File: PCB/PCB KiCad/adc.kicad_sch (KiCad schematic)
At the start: 10 parts, among them U2 NAU7802SGI, U4 LP5951MFX-1.8_NOPB

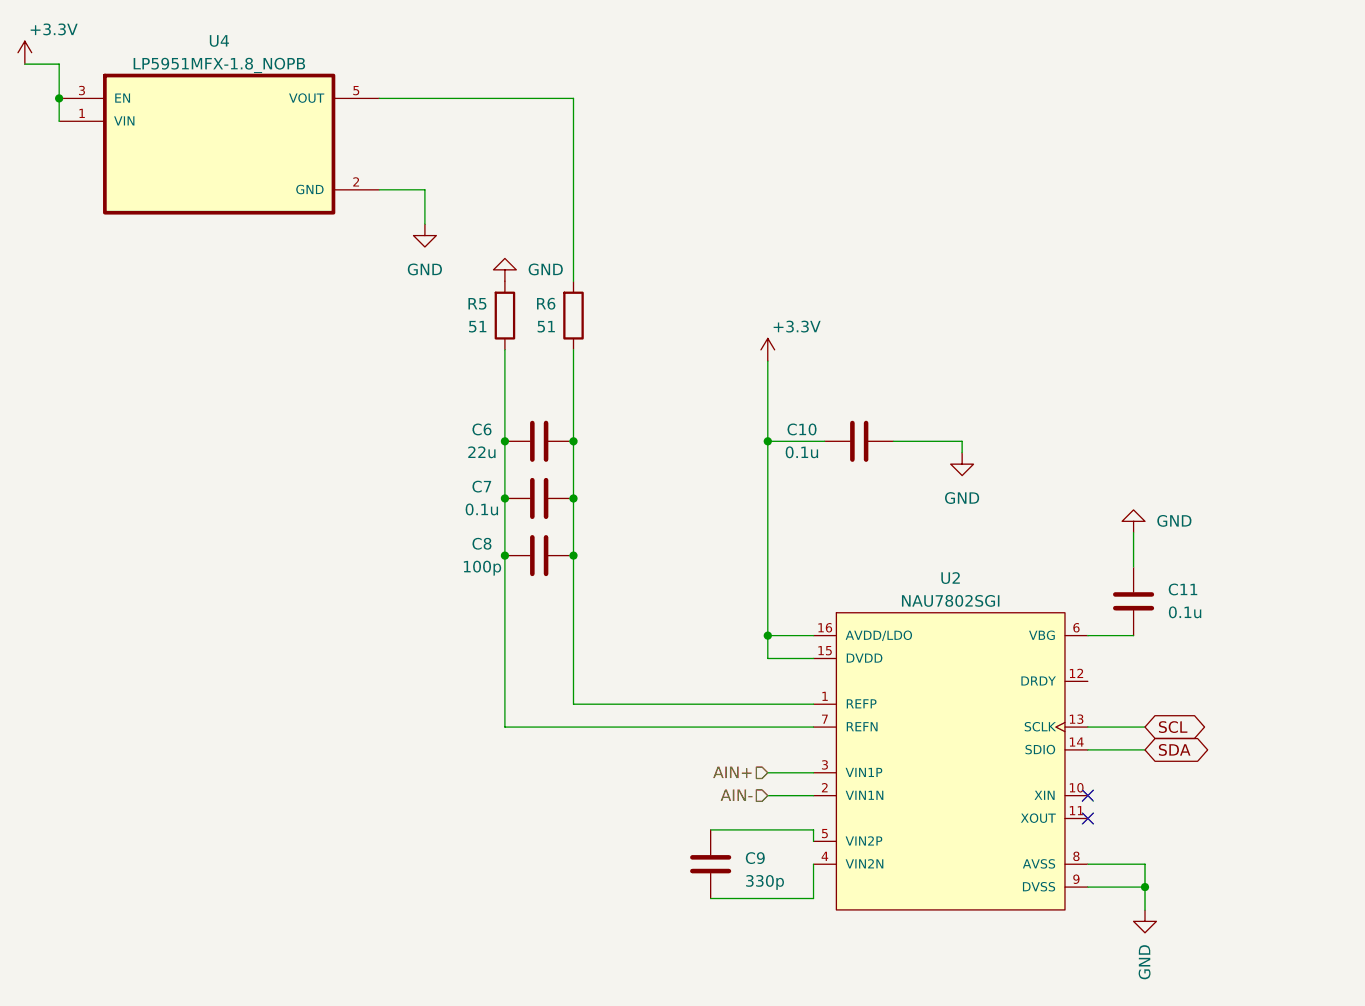
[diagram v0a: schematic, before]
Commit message: Minor schematic cleanup!
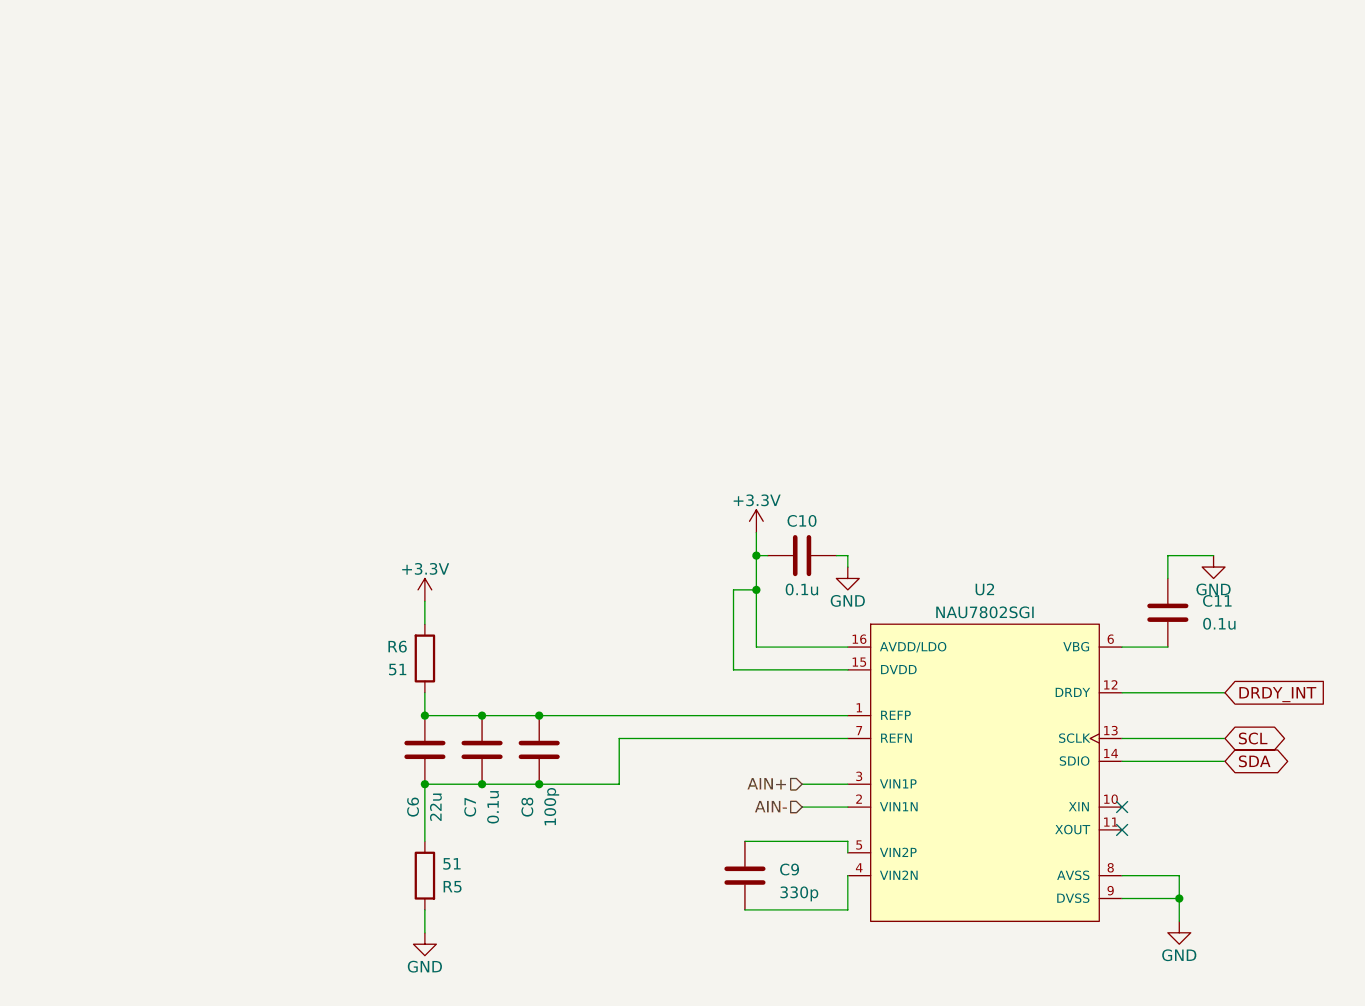
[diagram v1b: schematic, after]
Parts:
- removed U4: LP5951MFX-1.8_NOPB, LP5951MFX-1.8_NOPB:SOT95P280X145-5N, symbol LP5951MFX-1.8_NOPB:LP5951MFX-1.8_NOPB
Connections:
- net +3V3 is gone; now on net +3.3V: C10.1, U2.15 (DVDD), U2.16 (AVDD/LDO)
- net +3.3V: now reaches R6.2
- net DRDY_INT: now reaches U2.12 (DRDY)
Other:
- moved on the sheet: C10, C11, C6, C7, C8, C9, R5, R6, U2
